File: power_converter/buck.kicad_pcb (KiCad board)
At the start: 4 copper layers, 113.5 x 84 mm, 50 parts, among them J1 Conn_01x01, J2 Conn_01x01, Q1 Q_PMOS_GDS, U1 LTC2946CMS#PBF

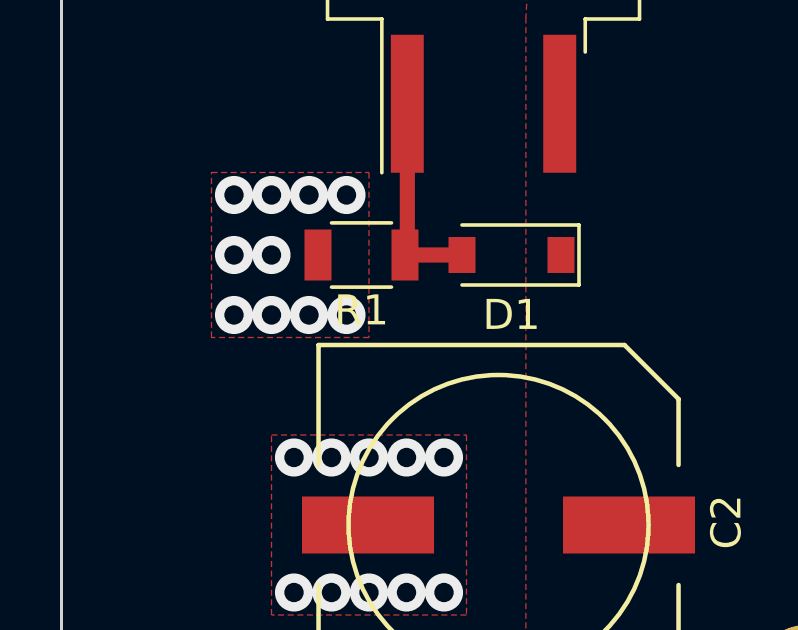
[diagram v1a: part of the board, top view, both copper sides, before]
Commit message: not much
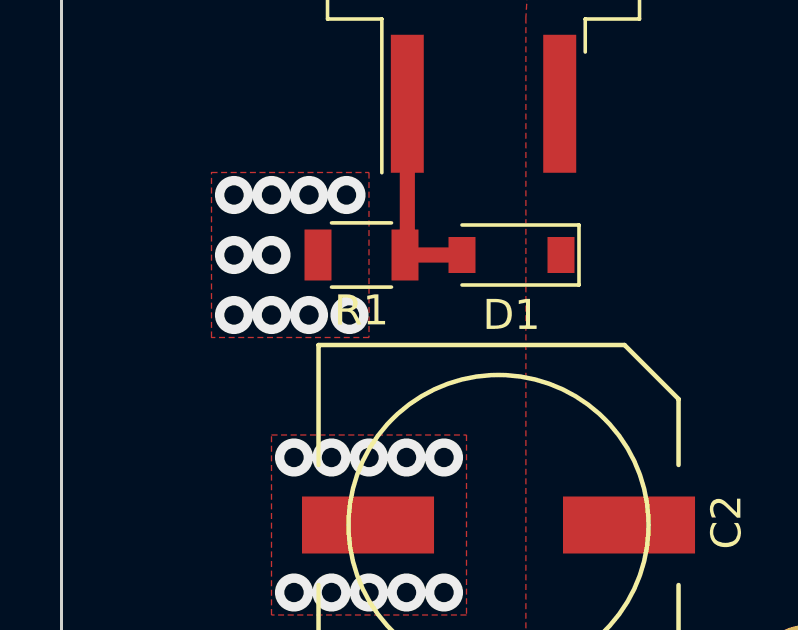
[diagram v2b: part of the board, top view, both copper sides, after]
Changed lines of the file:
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@@
   (layers
     (0 F.Cu signal)
-    (1 In1.Cu power hide)
-    (2 In2.Cu power hide)
+    (1 In1.Cu power)
+    (2 In2.Cu power)
     (31 B.Cu signal)
     (32 B.Adhes user)
@@
   (via (at 22 63) (size 1.27) (drill 0.64516) (layers F.Cu B.Cu) (net 1))
   (via (at 23.25 63) (size 1.27) (drill 0.64516) (layers F.Cu B.Cu) (net 1))
-  (via (at 24.5 63) (size 1.27) (drill 0.64516) (layers F.Cu B.Cu) (net 1))
+  (via (at 24.6 63) (size 1.27) (drill 0.64516) (layers F.Cu B.Cu) (net 1))
   (via (at 23.25 59) (size 1.27) (drill 0.64516) (layers F.Cu B.Cu) (net 1))
   (via (at 24.5 59) (size 1.27) (drill 0.64516) (layers F.Cu B.Cu) (net 1))
